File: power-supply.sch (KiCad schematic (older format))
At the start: 0 parts

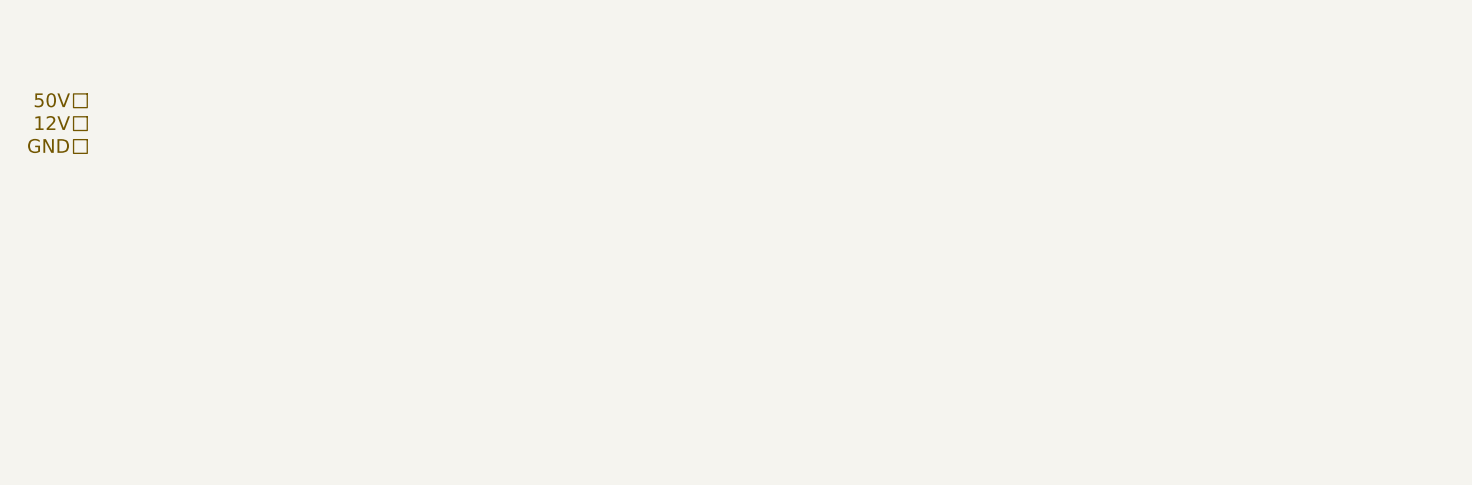
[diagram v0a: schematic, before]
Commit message: did the power sheet
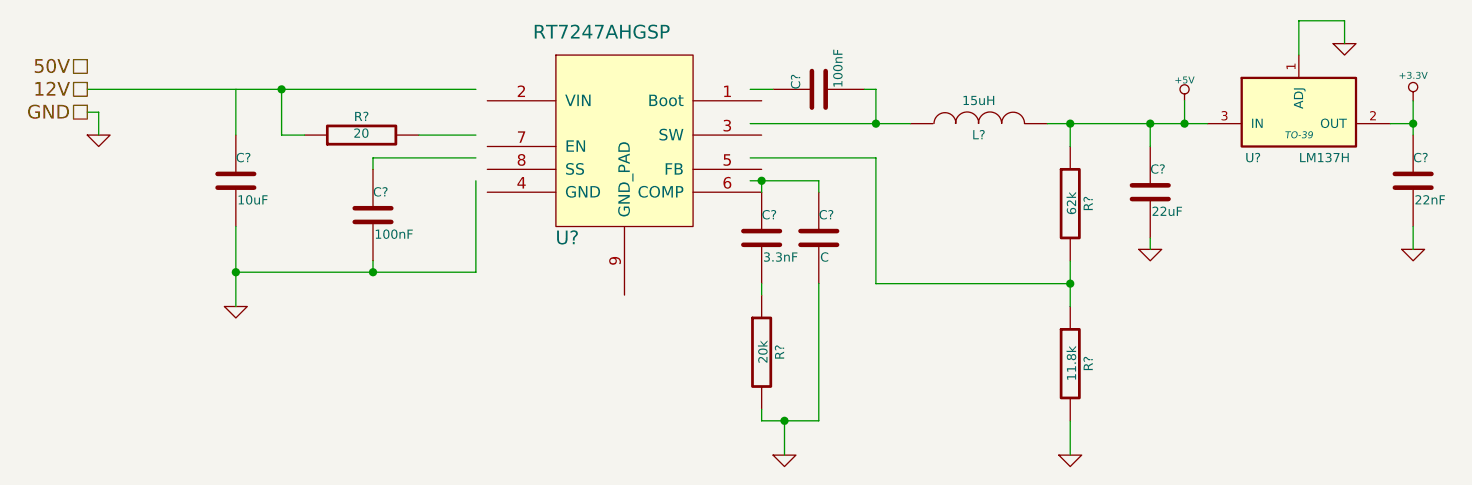
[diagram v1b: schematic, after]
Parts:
- added C?: 10uF, ~, symbol C
- added C? (x2): 100nF, ~, symbol C
- added C?: 3.3nF, ~, symbol C
- added C?: C, ~, symbol C
- added C?: 22uF, ~, symbol C
- added C?: 22nF, ~, symbol C
- added L?: 15uH, ~, symbol INDUCTOR
- added R?: 62k, ~, symbol R
- added R?: 11.8k, ~, symbol R
- added R?: 20k, ~, symbol R
- added R?: 20, ~, symbol R
- added U?: RT7247AHGSP, symbol RT7247AHGSP
- added U?: LM137H, TO-39, symbol LM137H
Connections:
- net labels added: +3.3V, +5V
- wire segments 0 -> 41
